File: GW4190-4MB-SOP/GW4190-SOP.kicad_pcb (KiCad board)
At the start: 4 copper layers, 88.9 x 20.3 mm, 10 parts, among them J1 DRAM-SIMM-30, U1 4C4M4, U2 4C4M4

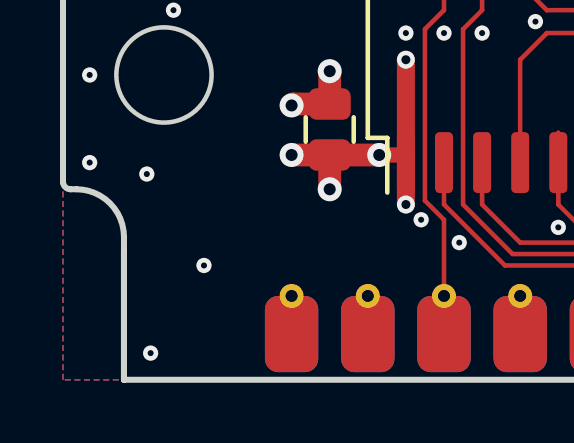
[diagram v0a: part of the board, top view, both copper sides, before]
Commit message: Fabbed
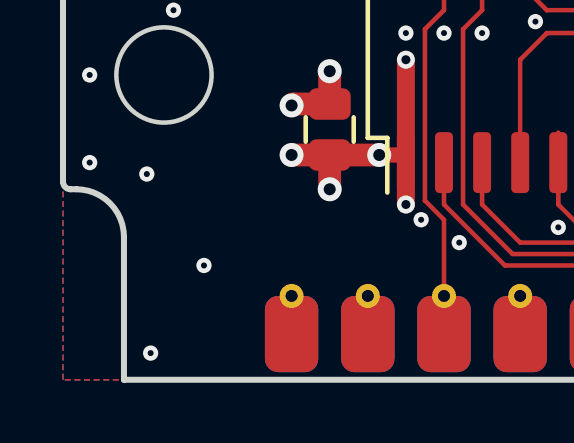
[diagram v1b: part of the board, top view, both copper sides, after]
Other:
- outline, holes or cut-outs redrawn
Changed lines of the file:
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@@
   (general
     (thickness 1.6)
-    (drawings 18)
+    (drawings 17)
     (tracks 536)
     (zones 0)
@@
     )
   )
+  (gr_line (start 78.232 101.6) (end 78.232 96.8375) (layer Edge.Cuts) (width 0.2))
   (gr_text "ZK, GF" (at 161.798 99.822) (layer B.SilkS)
     (effects (font (size 0.8128 0.8128) (thickness 0.2032)) (justify mirror))
@@
   (gr_arc (start 76.6445 96.8375) (end 78.232 96.8375) (angle -90) (layer Edge.Cuts) (width 0.2))
   (gr_line (start 76.2 94.996) (end 76.2 82.804) (layer Edge.Cuts) (width 0.2))
-  (gr_line (start 78.232 101.6) (end 78.232 96.8375) (layer Edge.Cuts) (width 0.2))
   (gr_line (start 76.6445 95.25) (end 76.454 95.25) (layer Edge.Cuts) (width 0.2))
   (gr_arc (start 76.454 94.996) (end 76.2 94.996) (angle -90) (layer Edge.Cuts) (width 0.2))
@@
     (effects (font (size 1.524 1.524) (thickness 0.3)) (justify mirror))
   )
-  (gr_line (start 78.232 101.6) (end 78.232 97.282) (layer Edge.Cuts) (width 0.2))
   (gr_circle (center 79.5655 91.44) (end 77.978 91.44) (layer Edge.Cuts) (width 0.15))
   (gr_circle (center 161.7345 91.44) (end 163.322 91.44) (layer Edge.Cuts) (width 0.15))
